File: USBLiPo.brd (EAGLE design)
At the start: 31.8 x 15.2 mm, 11 parts, among them IC1 LTC4054, J1 USB, J2 Li cell, Q1 2N7002

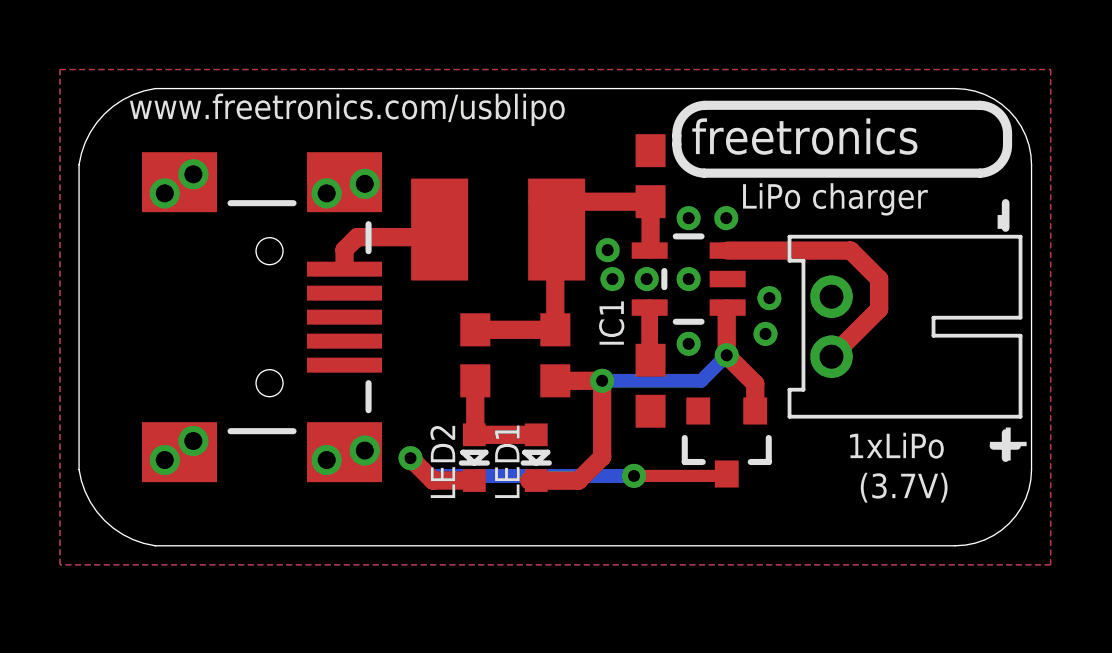
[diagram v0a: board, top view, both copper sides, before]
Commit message: foo
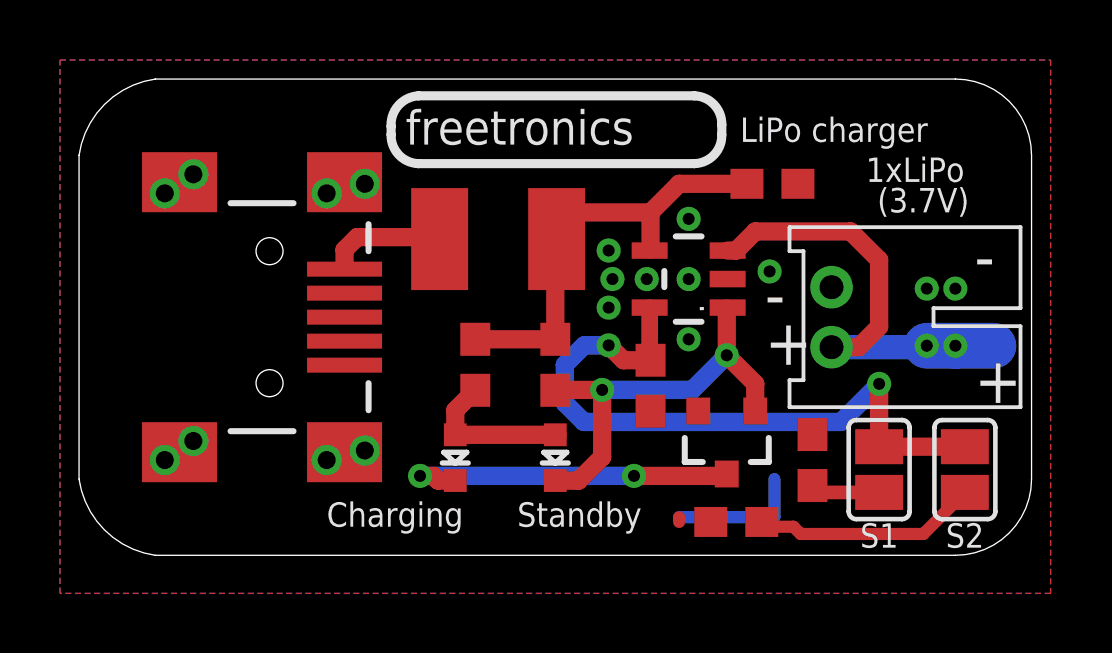
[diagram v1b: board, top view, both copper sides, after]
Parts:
- removed J2: Li cell, adafruit:JST-PH-2-THM-RA
- added B1: LiPo cell, freetronics-luke:JST-2MM-TH-RA
- added R4, R5: 10k, freetronics:0603
- added S1, S2: SJ, freetronics-luke:SJ
- LED1: value Green -> Charge
- LED2: value Red -> Standby
- R3: value 5.6k -> 3k3
- moved R3 5.94 mm to (24.4, 2.86), turned to 90 degrees
- moved C1 4.07 mm to (23.1, 12.1), turned to 180 degrees
- moved LED1 0.63 mm to (15.9, 2.94)
- moved LED2 0.63 mm to (12.5, 2.94)
- moved F1 0.32 mm to (14.0, 10.2)
- moved R1 0.32 mm to (13.2, 6.03)
- moved R2 0.32 mm to (15.9, 6.03)
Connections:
- new net N$5: R3.1, S1.1
- new net N$7: R4.1, S2.1
- net GND: now also B1.-, R4.2, R5.2; no longer J2.2
- net N$3: now also R5.1, S1.2, S2.2; no longer R3.1
- net N$4: now also B1.+; no longer J2.1
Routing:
- net N$3: track 1.77 -> 22.6 mm, vias 0 -> 2
- net N$7: track 0.00 -> 7.49 mm
- net N$4: track 8.69 -> 15.2 mm, vias 0 -> 2
- net GND: track 0.00 -> 4.60 mm, vias 17 -> 18
- net N$2: track 14.0 -> 17.8 mm
- net N$5: track 0.00 -> 2.28 mm
- net N$1: track 13.3 -> 11.5 mm
- net N$8: track 3.88 -> 5.25 mm
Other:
- board size 31.8 x 15.2 mm -> 31.8 x 15.9 mm
- board text added: "+"
- board text added: "-"
- board text added: "0 0 100 mA"
- board text added: "0 1 200 mA"
- board text added: "0= open"
- board text added: "1 0 303 mA"
- board text added: "1 1 503 mA"
- board text added: "1= short"
- board text added: "Charging"
- board text added: "S1"
- board text added: "S1 S2 Charge Current"
- board text added: "S2"
- board text added: "Standby"
